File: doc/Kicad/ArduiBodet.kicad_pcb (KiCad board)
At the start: 2 copper layers, 80 x 49.5 mm, 15 parts, among them CON1 BARREL_JACK, IC1 ATMEGA328-P, IC2 SN754410, P1 ISP10PIN, P2 DS3231_Breakout_Connector, P3 Moteur Horloge, SW1 SWITCH_INV, SW2 Switch_DPST

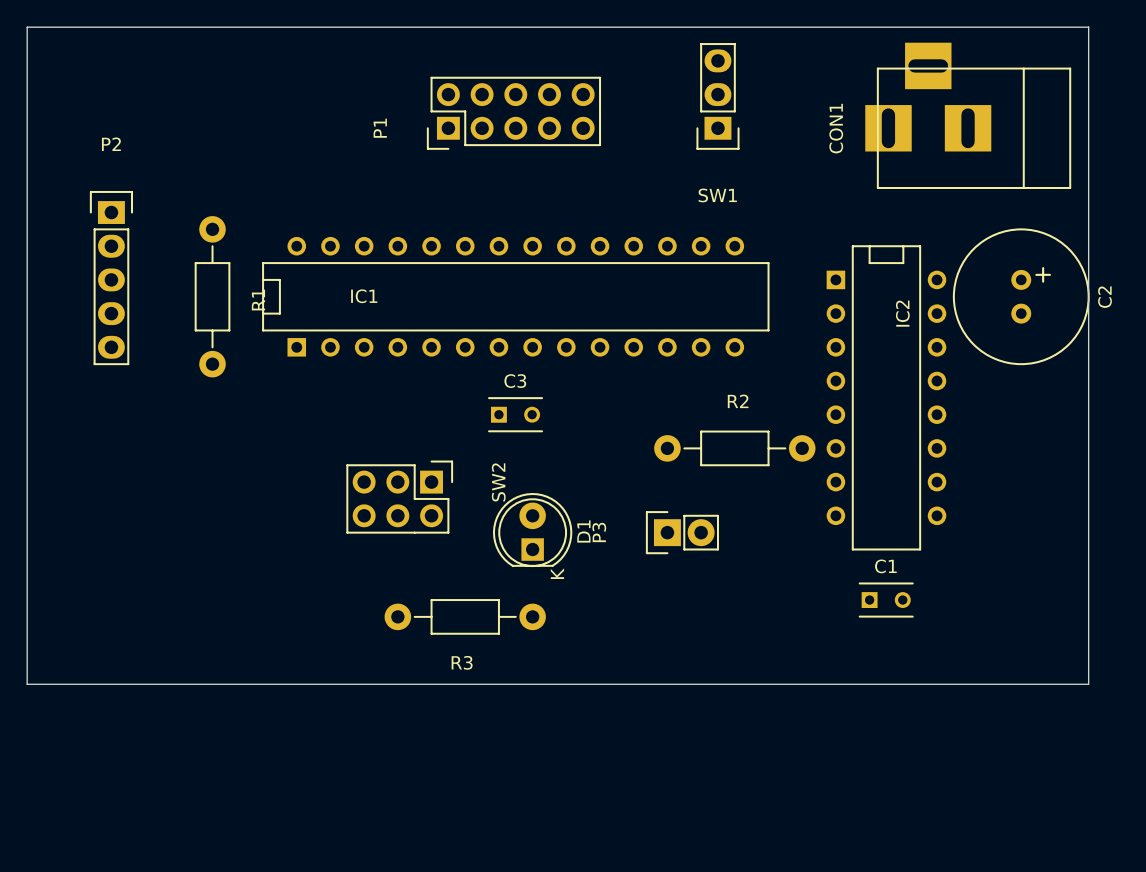
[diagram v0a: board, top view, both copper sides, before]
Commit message: routing in progress
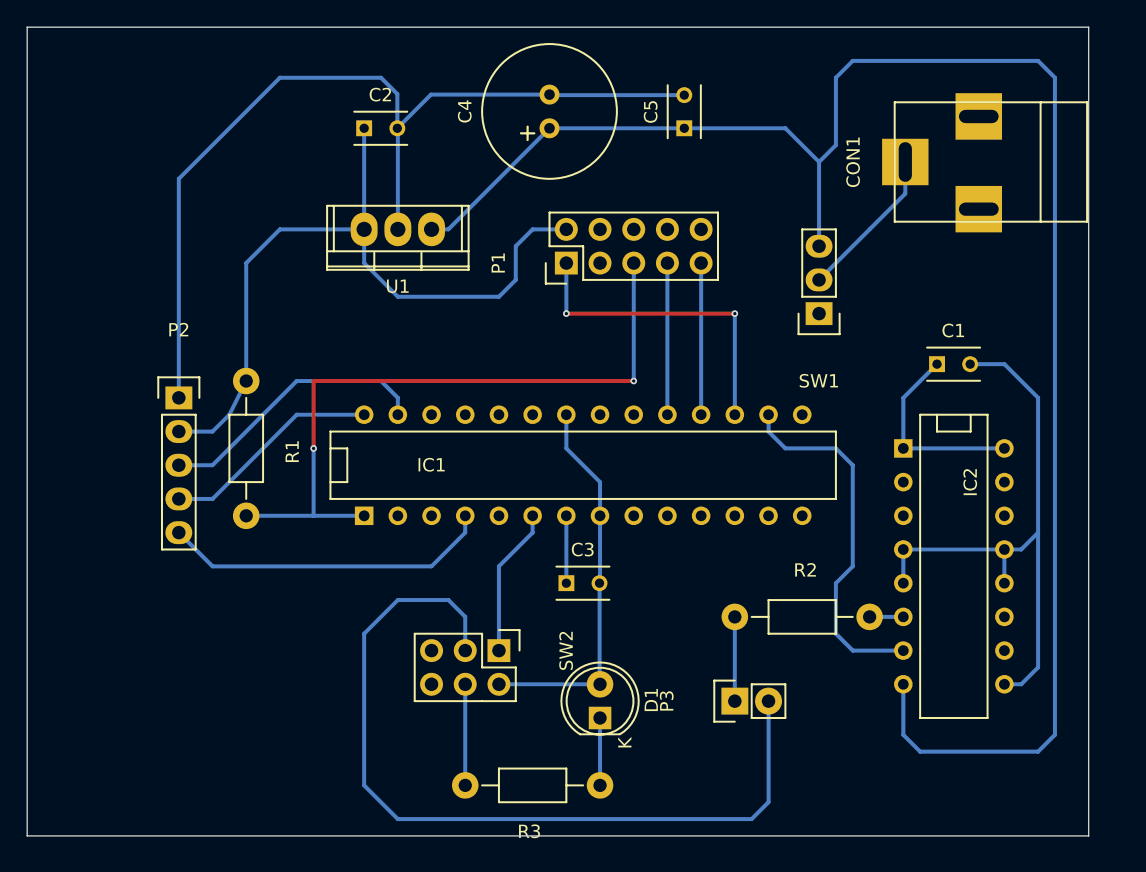
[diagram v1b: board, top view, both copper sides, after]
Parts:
- added C4: 1000 uF, Capacitors_Elko_ThroughHole:Elko_vert_20x10mm_RM2.5, F.Cu at (157.5, 95.2)
- added C5: 330nF, Capacitors_ThroughHole:C_Rect_L4_W2.5_P2.5, F.Cu at (167.6, 95.2)
- added U1: LM7805CT, Power_Integrations:TO-220, F.Cu at (146.1, 102.9)
- C2: value CP -> 100 nF; footprint Capacitors_Elko_ThroughHole:Elko_vert_20x10mm_RM2.5 -> Capacitors_ThroughHole:C_Rect_L4_W2.5_P2.5
- CON1: footprint Connect:BARREL_JACK -> myLib:BARREL_JACK_FR
- moved C2 50.8 mm to (143.5, 95.2), turned to 0 degrees
- moved C1 18.5 mm to (186.7, 113.0)
- moved SW1 15.9 mm to (177.8, 109.2)
- moved P2 14.9 mm to (129.5, 115.6)
- moved IC2 13.7 mm to (188.0, 128.3)
- moved R2 13.7 mm to (176.5, 132.1)
- moved IC1 13.7 mm to (160.0, 120.7)
- moved P3 13.7 mm to (171.4, 138.4)
- moved SW2 13.7 mm to (153.7, 134.6)
- moved C3 13.7 mm to (158.8, 129.5)
- moved R3 13.7 mm to (156.2, 144.8)
- moved D1 13.7 mm to (161.3, 139.7)
- moved P1 13.5 mm to (158.8, 105.4)
- moved R1 11.7 mm to (134.6, 119.4)
- moved CON1 2.84 mm to (190.5, 97.8)
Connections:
- CON1 pad 2: GNDA -> Net-(CON1-Pad2)
- CON1 pad 3: Net-(CON1-Pad3) -> GNDA
- IC2 pad 8: Net-(C1-Pad1) -> Net-(C4-Pad1)
- SW1 pad 1: Net-(C1-Pad1) -> Net-(SW1-Pad1)
- SW1 pad 3: Net-(SW1-Pad3) -> Net-(C4-Pad1)
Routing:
- net GNDA: track 0.00 -> 143.9 mm
- net Net-(C4-Pad1): track 0.00 -> 130.0 mm
- net Net-(C1-Pad1): track 0.00 -> 76.2 mm
- net Net-(IC2-Pad3): track 0.00 -> 62.8 mm
- net Net-(IC1-Pad1): track 0.00 -> 52.1 mm, vias 0 -> 2
- net Net-(IC1-Pad16): track 0.00 -> 27.5 mm
- net Net-(IC1-Pad4): track 0.00 -> 25.0 mm
- net Net-(IC1-Pad17): track 0.00 -> 24.1 mm, vias 0 -> 2
- net Net-(IC1-Pad27): track 0.00 -> 20.9 mm
- net Net-(IC1-Pad28): track 0.00 -> 16.6 mm
- net Net-(CON1-Pad1): track 0.00 -> 11.6 mm
- net Net-(IC1-Pad19): track 0.00 -> 11.4 mm
- net Net-(IC1-Pad18): track 0.00 -> 11.4 mm
- net Net-(IC1-Pad6): track 0.00 -> 11.2 mm
- net Net-(R3-Pad2): track 0.00 -> 7.62 mm
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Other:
- board size 80 x 49.5 mm -> 80 x 61 mm
